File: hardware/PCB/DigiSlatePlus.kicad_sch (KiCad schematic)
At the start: 48 parts, among them J4 USB_B, Q1 2N2222, U1 ESP32-S3-WROOM-1, U10 SA15-11SRWA, U11 KA78M05_TO252, U12 LM2596S-ADJ, U13 LD1117S33TR_SOT223, U14 DW01A, U2 MAX7219, U3 SA15-11SRWA, U4 SA15-11SRWA, U5 SA15-11SRWA, U6 SA15-11SRWA, U7 SA15-11SRWA, U8 SA15-11SRWA, U9 SA15-11SRWA

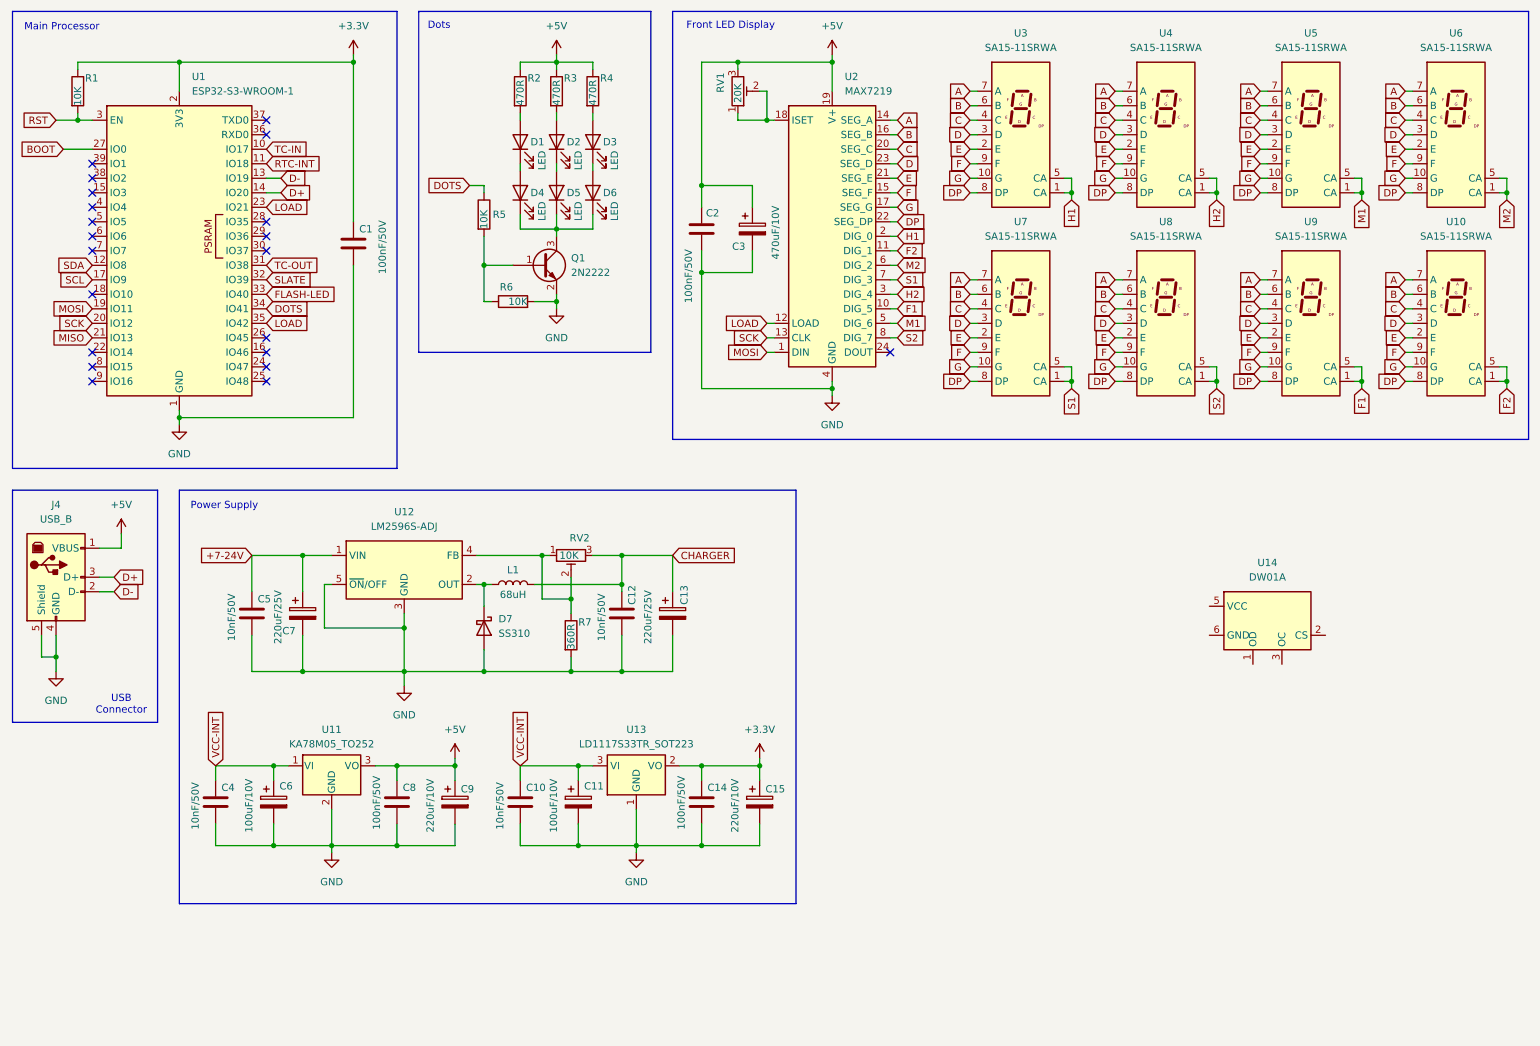
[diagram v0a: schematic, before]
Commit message: Schematic updated
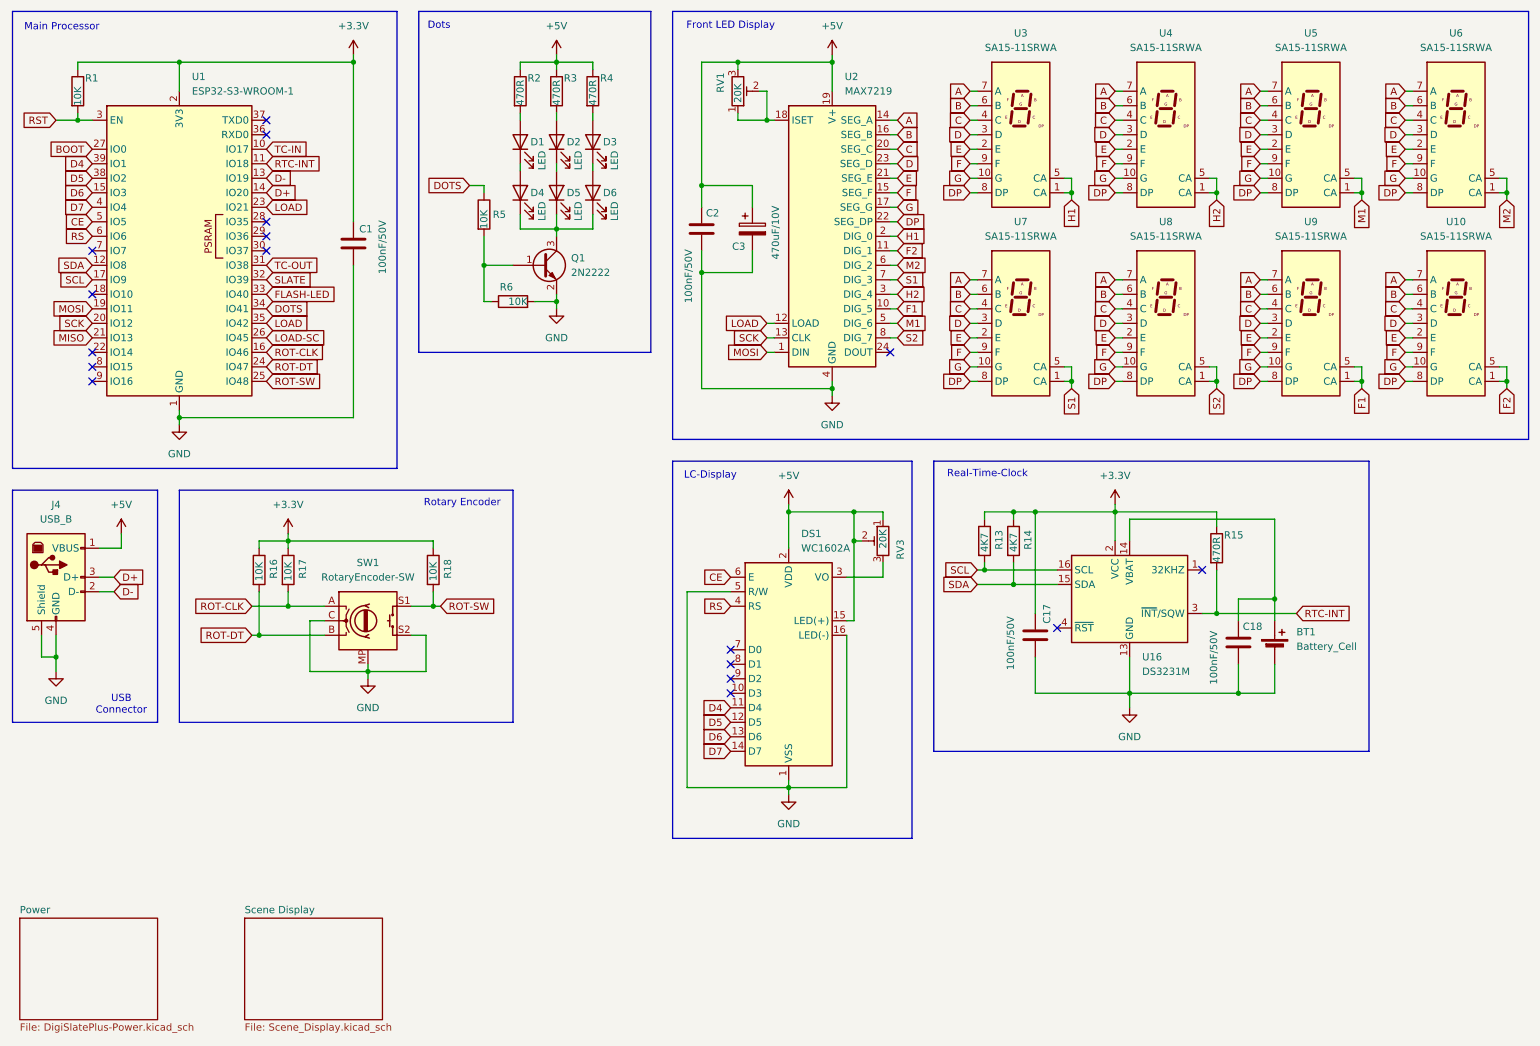
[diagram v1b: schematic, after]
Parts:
- removed C10, C12, C4, C5: 10nF/50V, Capacitor_SMD:C_1206_3216Metric_Pad1.33x1.80mm_HandSolder, symbol Device:C
- removed C11, C6: 100uF/10V, Capacitor_Tantalum_SMD:CP_EIA-7343-31_Kemet-D_Pad2.25x2.55mm_HandSolder, symbol Device:C_Polarized
- removed C13, C7: 220uF/25V, Capacitor_Tantalum_SMD:CP_EIA-7343-31_Kemet-D_Pad2.25x2.55mm_HandSolder, symbol Device:C_Polarized
- removed C14, C8: 100nF/50V, Capacitor_SMD:C_1206_3216Metric_Pad1.33x1.80mm_HandSolder, symbol Device:C
- removed C15, C9: 220uF/10V, Capacitor_Tantalum_SMD:CP_EIA-7343-31_Kemet-D_Pad2.25x2.55mm_HandSolder, symbol Device:C_Polarized
- removed D7: SS310, Diode_SMD:D_SMA, symbol Diode:SS310
- removed L1: 68uH, Inductor_SMD:L_7.3x7.3_H3.5, symbol Device:L
- removed R7: 360R, Resistor_SMD:R_1206_3216Metric, symbol Device:R
- removed RV2: 10K, Potentiometer_THT:Potentiometer_Bourns_3296W_Vertical, symbol Device:R_Potentiometer_Trim
- removed U11: KA78M05_TO252, Package_TO_SOT_SMD:TO-252-2, symbol Regulator_Linear:KA78M05_TO252
- removed U12: LM2596S-ADJ, Package_TO_SOT_SMD:TO-263-5_TabPin6, symbol Regulator_Switching:LM2596S-ADJ
- removed U13: LD1117S33TR_SOT223, Package_TO_SOT_SMD:SOT-223-3_TabPin2, symbol Regulator_Linear:LD1117S33TR_SOT223
- removed U14: DW01A, Package_TO_SOT_SMD:SOT-23-6, symbol Battery_Management:DW01A
- added BT1: Battery_Cell, Battery:BatteryHolder_ComfortableElectronic_CH273-2450_1x2450, symbol Device:Battery_Cell
- added C17, C18: 100nF/50V, Capacitor_SMD:C_1206_3216Metric_Pad1.33x1.80mm_HandSolder, symbol Device:C
- added DS1: WC1602A, Display:WC1602A, symbol 7-Segment:WC1602A
- added R13, R14: 4K7, Resistor_SMD:R_1206_3216Metric, symbol Device:R
- added R15: 470R, Resistor_SMD:R_1206_3216Metric, symbol Device:R
- added R16, R17, R18: 10K, Resistor_SMD:R_1206_3216Metric, symbol Device:R
- added RV3: 20K, Potentiometer_SMD:Potentiometer_Vishay_TS53YL_Vertical, symbol Device:R_Potentiometer_Trim
- added SW1: RotaryEncoder-SW, Rotary_Encoder:RotaryEncoder_Bourns_Horizontal_PEC12R-2x17F-Sxxxx, symbol Device:RotaryEncoder_Switch_MP
- added U16: DS3231M, Package_SO:SOIC-16W_7.5x10.3mm_P1.27mm, symbol Timer_RTC:DS3231M
- J4: footprint (none) -> Connector_USB:USB_B_Lumberg_2411_02_Horizontal
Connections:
- net +3.3V: now also C17.1, R13.1, R14.1, R15.1, R16.1, R17.1, R18.1, U16.2 (VCC)
- net +5V: now also DS1.15 (LED(+)), DS1.2 (VDD), RV3.1, RV3.2
- net GND: now also BT1.2 (-), C17.2, C18.2, DS1.1 (VSS), DS1.16 (LED(-)), DS1.5 (R/W), SW1.C, SW1.MP, SW1.S2, U16.10 (GND), U16.11 (GND), U16.12 (GND), U16.13 (GND), U16.5 (GND), U16.6 (GND), U16.7 (GND), U16.8 (GND), U16.9 (GND)
- net RTC-INT: now also R15.2, U16.3 (~{INT}/SQW)
- net SCL: now also R13.2, U16.16 (SCL)
- net SDA: now also R14.2, U16.15 (SDA)
- net D6: now reaches U1.15 (IO3)
- net D6: now also DS1.13 (D6)
- net ROT-CLK: now reaches U1.16 (IO46)
- net ROT-CLK: now also R17.2, SW1.A
- net ROT-DT: now reaches U1.24 (IO47)
- net ROT-DT: now also R16.2, SW1.B
- net ROT-SW: now reaches U1.25 (IO48)
- net ROT-SW: now also R18.2, SW1.S1
- net LOAD-SC: now reaches U1.26 (IO45)
- net D5: now reaches U1.38 (IO2)
- net D5: now also DS1.12 (D5)
- net D4: now reaches U1.39 (IO1)
- net D4: now also DS1.11 (D4)
- net D7: now reaches U1.4 (IO4)
- net D7: now also DS1.14 (D7)
- net CE: now reaches U1.5 (IO5)
- net CE: now also DS1.6 (E)
- net RS: now reaches U1.6 (IO6)
- net RS: now also DS1.4 (RS)
- new net: DS1.3 (VO), RV3.3
- new net: BT1.1 (+), C18.1, U16.14 (VBAT)
- no-connect marks 21 -> 17
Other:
- added sheet Power (DigiSlatePlus-Power.kicad_sch)
- added sheet Scene Display (Scene_Display.kicad_sch)
- note added: "LC-Display"
- note added: "Real-Time-Clock"
- note added: "Rotary Encoder"
- note removed: "Power Supply"
